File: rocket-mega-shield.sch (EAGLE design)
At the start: 66 parts, among them J1 ExtBatt, J2 Mega R3, J3 XBEE, J4 MICROSD, J5 U.FL, J6 1X6TERMINALBLOCK, Q1 SI7112DN, Q2 BSS138, Q3 BSS138, Q4 SI7112DN, Q5 SI7112DN, Q6 SI7112DN, Q7 SI7112DN, U1 NCP1117DT33G, U2 M74HC4050M, U3 FGPMMOPA6H, U4 BMP180, U5 LSM303DLHCTR, U6 L3GD20TR, U7 ADXL377

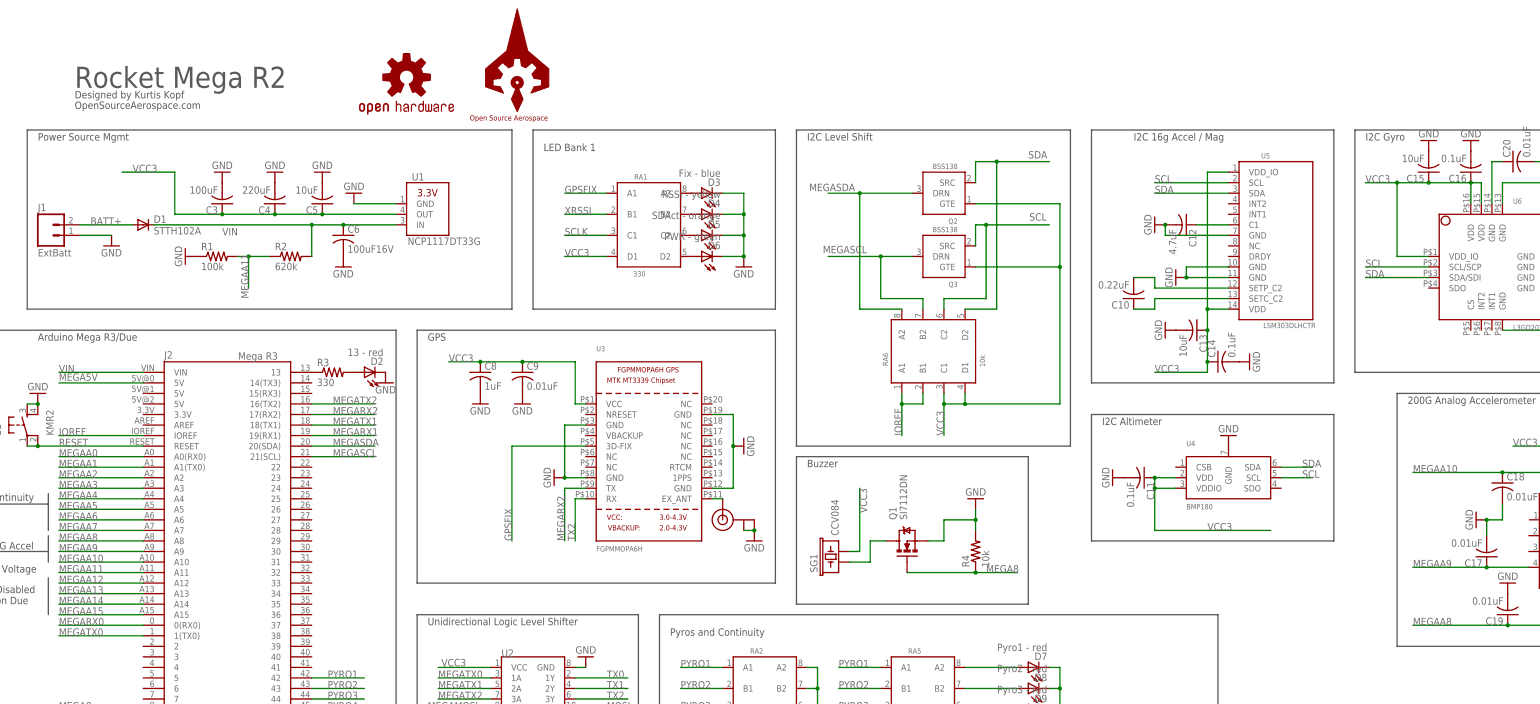
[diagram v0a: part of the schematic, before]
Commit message: more cleanup on the 2.1 board
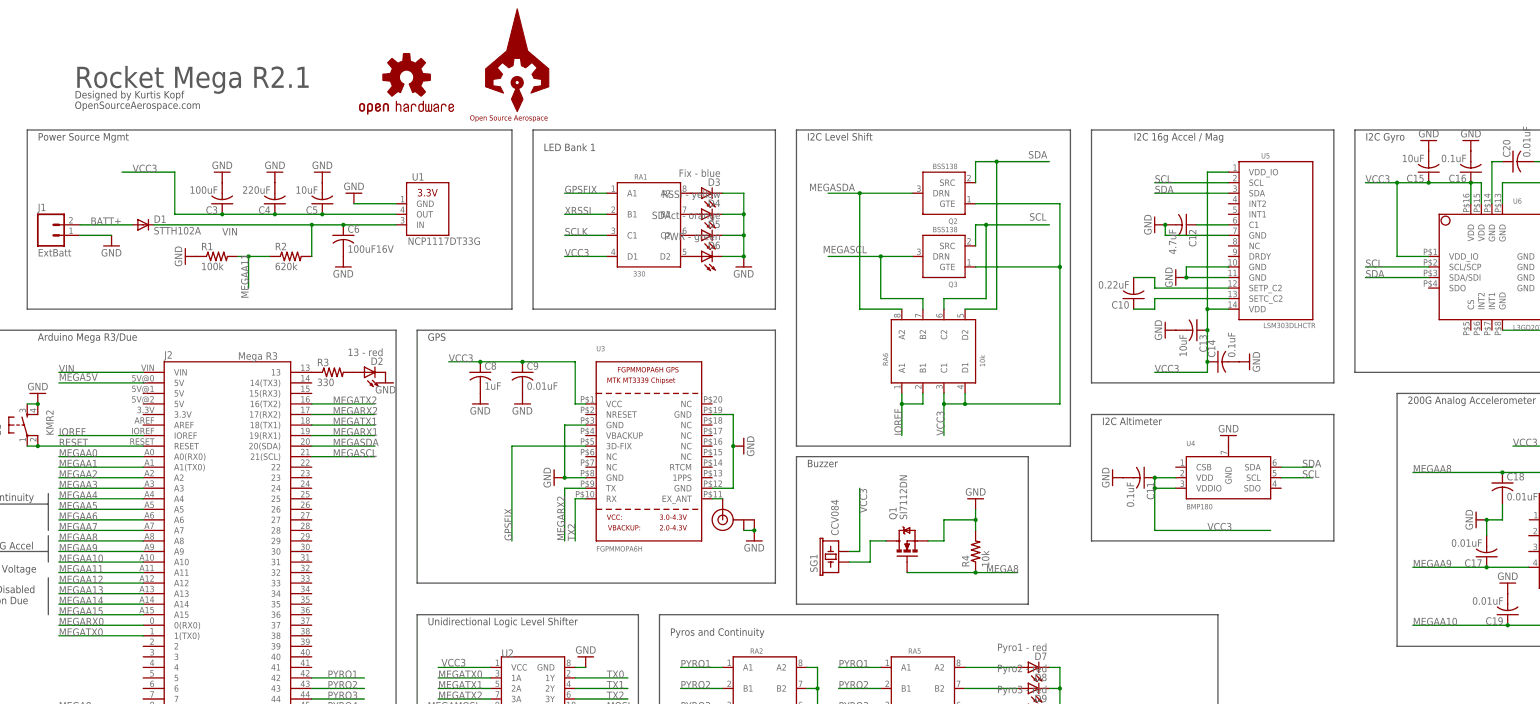
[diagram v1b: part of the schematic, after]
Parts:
- Q1, Q4, Q5, Q6, Q7: device SparkFun-DiscreteSemi:MOSFET-NCHANNELSI7820DN -> zortness:MOSFET-NCHANNELSI7820DN
- U1: device kurt:NCP1117DT33G -> zortness:NCP1117DT33G
- U3: device adafruit:GPS_FGPMMOPA6H -> zortness:GPS_FGPMMOPA6H
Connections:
- net MEGAA10: now also C19.1, U7.X; no longer C18.1, U7.Z
- net MEGAA8: now also C18.1, U7.Z; no longer C19.1, U7.X
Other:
- note added: "Rocket Mega R2.1"
- note removed: "Rocket Mega R2"
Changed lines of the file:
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@@
 <part name="J3" library="zortness" deviceset="XBEE" device=""/>
 <part name="J4" library="zortness" deviceset="MICROSD" device=""/>
-<part name="U3" library="adafruit" deviceset="GPS_FGPMMOPA6H" device="" value="FGPMMOPA6H"/>
+<part name="U3" library="zortness" deviceset="GPS_FGPMMOPA6H" device="" value="FGPMMOPA6H"/>
 <part name="U6" library="kurt" deviceset="L3GD20" device="" value="L3GD20TR"/>
 <part name="U5" library="kurt" deviceset="LSM303DLHC" device="" value="LSM303DLHCTR"/>
-<part name="U1" library="kurt" deviceset="NCP1117DT33G" device=""/>
+<part name="U1" library="zortness" deviceset="NCP1117DT33G" device=""/>
 <part name="Q3" library="kurt" deviceset="BSS138" device="" value="BSS138"/>
 <part name="Q2" library="kurt" deviceset="BSS138" device="" value="BSS138"/>
@@
 <part name="U2" library="SparkFun-DigitalIC" deviceset="HEX_CONVERTER" device="" value="M74HC4050M"/>
 <part name="GND37" library="supply1" deviceset="GND" device=""/>
-<part name="Q7" library="SparkFun-DiscreteSemi" deviceset="MOSFET-NCHANNEL" device="SI7820DN" value="SI7112DN"/>
-<part name="Q4" library="SparkFun-DiscreteSemi" deviceset="MOSFET-NCHANNEL" device="SI7820DN" value="SI7112DN"/>
-<part name="Q6" library="SparkFun-DiscreteSemi" deviceset="MOSFET-NCHANNEL" device="SI7820DN" value="SI7112DN"/>
-<part name="Q5" library="SparkFun-DiscreteSemi" deviceset="MOSFET-NCHANNEL" device="SI7820DN" value="SI7112DN"/>
+<part name="Q7" library="zortness" deviceset="MOSFET-NCHANNEL" device="SI7820DN" value="SI7112DN"/>
+<part name="Q4" library="zortness" deviceset="MOSFET-NCHANNEL" device="SI7820DN" value="SI7112DN"/>
+<part name="Q6" library="zortness" deviceset="MOSFET-NCHANNEL" device="SI7820DN" value="SI7112DN"/>
+<part name="Q5" library="zortness" deviceset="MOSFET-NCHANNEL" device="SI7820DN" value="SI7112DN"/>
 <part name="U7" library="zortness" deviceset="ADXL377" device=""/>
 <part name="GND3" library="supply1" deviceset="GND" device=""/>
@@
 <part name="GND20" library="supply1" deviceset="GND" device=""/>
 <part name="LOGO1" library="SparkFun-Aesthetics" deviceset="OSHW-LOGO" device="M"/>
-<part name="Q1" library="SparkFun-DiscreteSemi" deviceset="MOSFET-NCHANNEL" device="SI7820DN" value="SI7112DN"/>
+<part name="Q1" library="zortness" deviceset="MOSFET-NCHANNEL" device="SI7820DN" value="SI7112DN"/>
 <part name="U$1" library="zortness" deviceset="OSAEROSPACE" device="VECTOR"/>
 </parts>
@@
 <wire x1="134.62" y1="-121.92" x2="134.62" y2="-2.54" width="0.1524" layer="97"/>
 <wire x1="134.62" y1="-2.54" x2="0" y2="-2.54" width="0.1524" layer="97"/>
-<text x="-140.97" y="124.46" size="5.08" layer="97">Rocket Mega R2</text>
+<text x="-140.97" y="124.46" size="5.08" layer="97">Rocket Mega R2.1</text>
 <wire x1="-30.48" y1="114.3" x2="-30.48" y2="71.12" width="0.1524" layer="97"/>
 <wire x1="-30.48" y1="71.12" x2="27.94" y2="71.12" width="0.1524" layer="97"/>
@@
 </segment>
 <segment>
+<pinref part="U7" gate="G$1" pin="Z"/>
+<wire x1="217.17" y1="29.21" x2="217.17" y2="31.75" width="0.1524" layer="91"/>
+<wire x1="217.17" y1="31.75" x2="203.2" y2="31.75" width="0.1524" layer="91"/>
+<pinref part="C18" gate="G$1" pin="1"/>
+<wire x1="203.2" y1="31.75" x2="181.61" y2="31.75" width="0.1524" layer="91"/>
+<junction x="203.2" y="31.75"/>
+<label x="181.61" y="31.75" size="1.778" layer="95"/>
+</segment>
+</net>
+<net name="MEGAA9" class="0">
+<segment>
+<pinref part="J2" gate="G$1" pin="A9"/>
+<wire x1="-124.46" y1="12.7" x2="-144.78" y2="12.7" width="0.1524" layer="91"/>
+<label x="-144.78" y="12.7" size="1.778" layer="95"/>
+</segment>
+<segment>
+<pinref part="U7" gate="G$1" pin="Y"/>
+<wire x1="209.55" y1="8.89" x2="199.39" y2="8.89" width="0.1524" layer="91"/>
+<pinref part="C17" gate="G$1" pin="1"/>
+<wire x1="199.39" y1="8.89" x2="181.61" y2="8.89" width="0.1524" layer="91"/>
+<junction x="199.39" y="8.89"/>
+<label x="181.61" y="8.89" size="1.778" layer="95"/>
+</segment>
+</net>
+<net name="MEGAA10" class="0">
+<segment>
+<pinref part="J2" gate="G$1" pin="A10"/>
+<wire x1="-124.46" y1="10.16" x2="-144.78" y2="10.16" width="0.1524" layer="91"/>
+<label x="-144.78" y="10.16" size="1.778" layer="95"/>
+</segment>
+<segment>
 <pinref part="U7" gate="G$1" pin="X"/>
 <wire x1="217.17" y1="1.27" x2="217.17" y2="-5.08" width="0.1524" layer="91"/>
@@
 </segment>
 </net>
-<net name="MEGAA9" class="0">
-<segment>
-<pinref part="J2" gate="G$1" pin="A9"/>
-<wire x1="-124.46" y1="12.7" x2="-144.78" y2="12.7" width="0.1524" layer="91"/>
-<label x="-144.78" y="12.7" size="1.778" layer="95"/>
-</segment>
-<segment>
-<pinref part="U7" gate="G$1" pin="Y"/>
-<wire x1="209.55" y1="8.89" x2="199.39" y2="8.89" width="0.1524" layer="91"/>
-<pinref part="C17" gate="G$1" pin="1"/>
-<wire x1="199.39" y1="8.89" x2="181.61" y2="8.89" width="0.1524" layer="91"/>
-<junction x="199.39" y="8.89"/>
-<label x="181.61" y="8.89" size="1.778" layer="95"/>
-</segment>
-</net>
-<net name="MEGAA10" class="0">
-<segment>
-<pinref part="J2" gate="G$1" pin="A10"/>
-<wire x1="-124.46" y1="10.16" x2="-144.78" y2="10.16" width="0.1524" layer="91"/>
-<label x="-144.78" y="10.16" size="1.778" layer="95"/>
-</segment>
-<segment>
-<pinref part="U7" gate="G$1" pin="Z"/>
-<wire x1="217.17" y1="29.21" x2="217.17" y2="31.75" width="0.1524" layer="91"/>
-<wire x1="217.17" y1="31.75" x2="203.2" y2="31.75" width="0.1524" layer="91"/>
-<pinref part="C18" gate="G$1" pin="1"/>
-<wire x1="203.2" y1="31.75" x2="181.61" y2="31.75" width="0.1524" layer="91"/>
-<junction x="203.2" y="31.75"/>
-<label x="181.61" y="31.75" size="1.778" layer="95"/>
-</segment>
-</net>
